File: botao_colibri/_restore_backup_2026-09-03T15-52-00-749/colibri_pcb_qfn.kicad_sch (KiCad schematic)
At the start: 10 parts, among them J2 TC2030, J5 Conn_01x06, J6 Conn_01x06, J7 Conn_01x02, J8 Conn_01x02, U1 ME54BS12

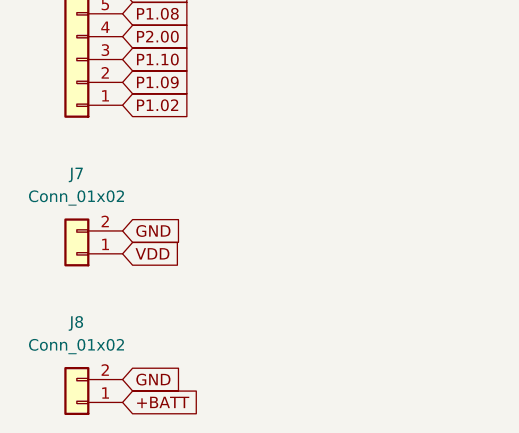
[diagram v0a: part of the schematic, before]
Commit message: Pedidos do henrique
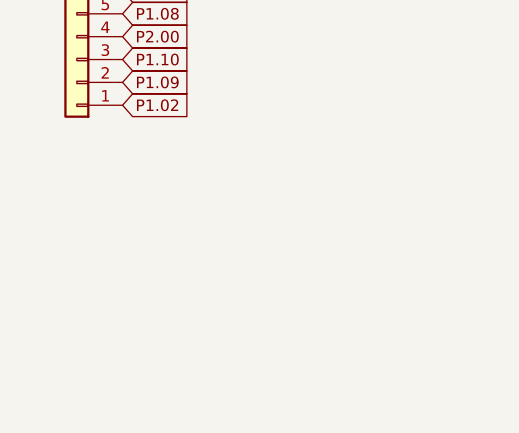
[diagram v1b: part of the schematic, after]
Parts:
- removed J7: Conn_01x02, Connector_PinHeader_2.54mm:PinHeader_1x02_P2.54mm_Vertical, symbol Connector_Generic:Conn_01x02
- removed J8: Conn_01x02, Connector_JST:JST_PH_S2B-PH-K_1x02_P2.00mm_Horizontal, symbol Connector_Generic:Conn_01x02
